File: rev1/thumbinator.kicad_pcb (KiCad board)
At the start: 2 copper layers, 45 x 20 mm, 16 parts, among them P1 CONN_02X06, P2 USB_A, P3 CONN_01X04, SW1 SW_PUSH, U1 AP1117D33, U2 STM32F072CBTx

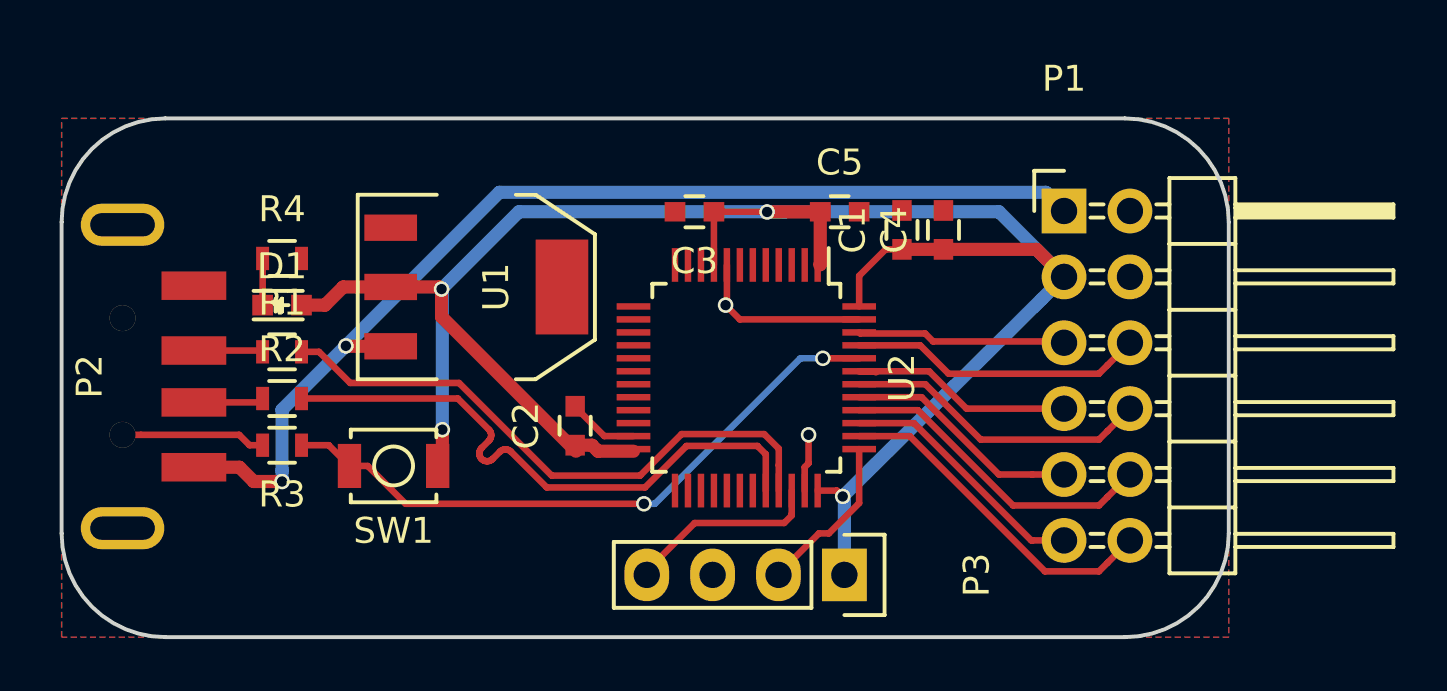
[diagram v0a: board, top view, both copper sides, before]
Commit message: PCB polishing
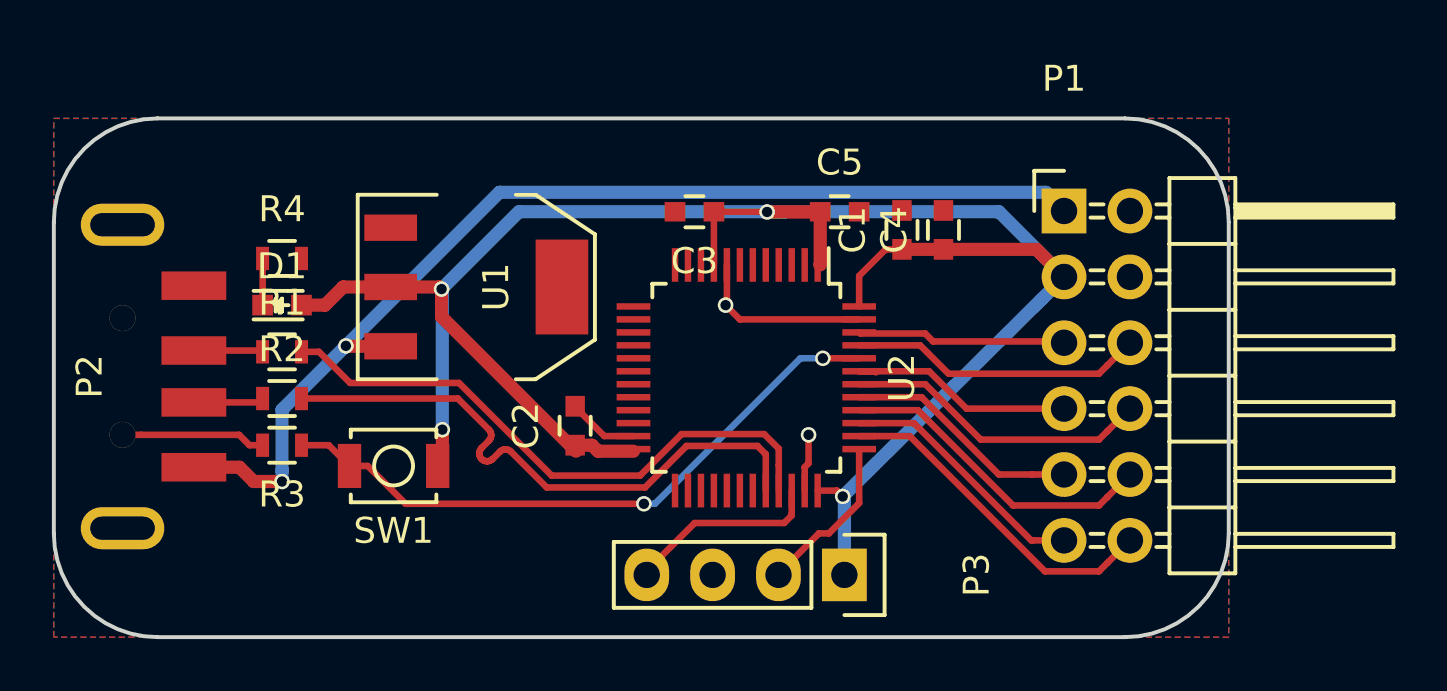
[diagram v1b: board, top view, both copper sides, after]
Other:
- board size 45 x 20 mm -> 45.3 x 20 mm
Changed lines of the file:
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@@
 (kicad_pcb (version 4) (host pcbnew 4.0.2-stable)
   (general
-    (links 52)
-    (no_connects 25)
-    (area 49.924999 49.924999 95.075001 70.075001)
+    (links 53)
+    (no_connects 0)
+    (area 49.624999 49.924999 95.075001 70.075001)
     (thickness 1.6)
     (drawings 8)
@@
     (pad 5 thru_hole circle (at 2.25 0 270) (size 1 1) (drill 1) (layers *.Cu *.Mask F.SilkS)
       (net 2 GND))
-    (model ../../../../../../Users/Konrad/hw/thumbinator-hw/3rd_party/models/usb_thruhole.wrl
+    (model ../../../../../../Users/Konrad/hw/thumbinator-hw/3rd_party/models/usb_smd.wrl
       (at (xyz 0 -0.33 0.025))
       (scale (xyz 0.393 0.393 0.393))
@@
   (gr_arc (start 91 66) (end 95 66) (angle 90) (layer Edge.Cuts) (width 0.15))
   (gr_arc (start 91 54) (end 91 50) (angle 90) (layer Edge.Cuts) (width 0.15))
-  (gr_arc (start 54 66) (end 54 70) (angle 90) (layer Edge.Cuts) (width 0.15))
-  (gr_arc (start 54 54) (end 50 54) (angle 90) (layer Edge.Cuts) (width 0.15))
-  (gr_line (start 50 66) (end 50 54) (layer Edge.Cuts) (width 0.15))
-  (gr_line (start 91 70) (end 54 70) (layer Edge.Cuts) (width 0.15))
+  (gr_arc (start 53.7 66) (end 53.7 70) (angle 90) (layer Edge.Cuts) (width 0.15))
+  (gr_arc (start 53.7 54) (end 49.7 54) (angle 90) (layer Edge.Cuts) (width 0.15))
+  (gr_line (start 49.7 66) (end 49.7 54) (layer Edge.Cuts) (width 0.15))
+  (gr_line (start 91 70) (end 53.7 70) (layer Edge.Cuts) (width 0.15))
   (gr_line (start 95 54) (end 95 66) (layer Edge.Cuts) (width 0.15))
-  (gr_line (start 54 50) (end 91 50) (layer Edge.Cuts) (width 0.15))
+  (gr_line (start 53.7 50) (end 91 50) (layer Edge.Cuts) (width 0.15))
   (segment (start 79.25 53.6) (end 79.25 55.632201) (width 0.508) (layer F.Cu) (net 1))
   (segment (start 79.25 55.632201) (end 79.232201 55.65) (width 0.508) (layer F.Cu) (net 1))
@@
     (polygon
       (pts
-        (xy 50 50) (xy 95 50) (xy 95 70) (xy 50 70)
+        (xy 49.7 50) (xy 95 50) (xy 95 70) (xy 49.7 70)
       )
     )
@@
     (polygon
       (pts
-        (xy 50 50) (xy 95 50) (xy 95 70) (xy 50 70)
+        (xy 49.7 50) (xy 95 50) (xy 95 70) (xy 49.7 70)
       )
     )

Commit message: Tweaking
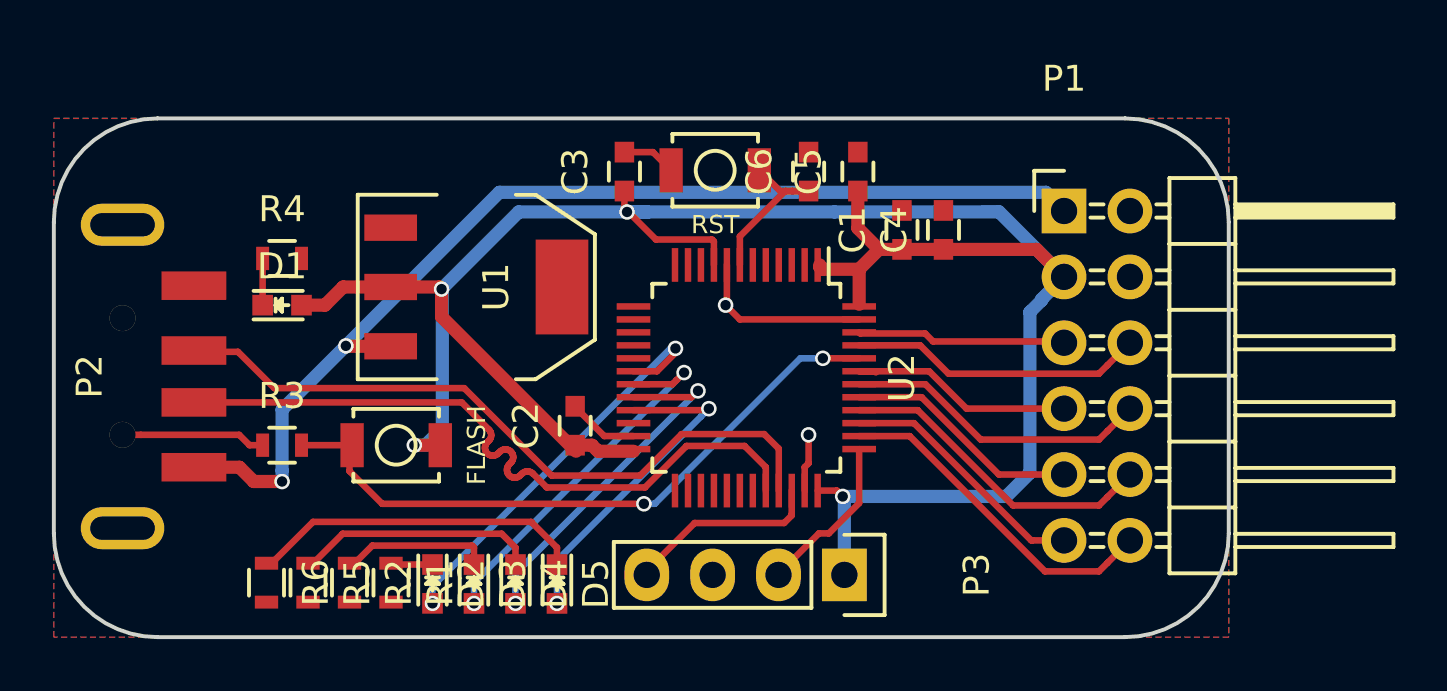
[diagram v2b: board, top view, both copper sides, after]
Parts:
- added C6: 100nF, Capacitors_SMD:C_0603, F.Cu at (78.8, 52.0)
- added D2: LED, LEDs:LED_0603, F.Cu at (64.3, 67.9)
- added D3: LED, LEDs:LED_0603, F.Cu at (65.9, 68.0)
- added D4: LED, LEDs:LED_0603, F.Cu at (67.5, 67.9)
- added D5: LED, LEDs:LED_0603, F.Cu at (69.1, 68.0)
- added R5: 360R, Resistors_SMD:R_0603, F.Cu at (59.5, 67.9)
- added R6: 360R, Resistors_SMD:R_0603, F.Cu at (57.9, 67.9)
- added SW2: SW_PUSH, Buttons_Switches_SMD:SW_SPST_B3U-1000P, F.Cu at (75.2, 52.0)
- R1, R2: value 47R -> 360R
- moved R1 9.84 mm to (62.7, 67.9), turned to 270 degrees
- moved R2 7.56 mm to (61.1, 67.9), turned to 270 degrees
- moved C3 3.11 mm to (71.7, 52.0), turned to 90 degrees
- moved C5 1.70 mm to (80.7, 52.0), turned to 90 degrees
- moved SW1 0.81 mm to (62.9, 62.6)
- turned R3 to 0 degrees
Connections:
- P2 pad 2: /USB_RAW_D- -> /STM32F072C8T6/USB_D-
- P2 pad 3: /USB_RAW_D+ -> /STM32F072C8T6/USB_D+
- R1 pad 1: /USB_RAW_D+ -> Net-(D2-Pad1)
- R1 pad 2: /STM32F072C8T6/USB_D+ -> GND
- R2 pad 1: /USB_RAW_D- -> Net-(D3-Pad1)
- R2 pad 2: /STM32F072C8T6/USB_D- -> GND
- R3 pad 1: /STM32F072C8T6/BOOT0 -> GND
- R3 pad 2: GND -> /STM32F072C8T6/BOOT0
- U1 pad 4: GND -> (no net)
- U2 pad 18: Net-(U2-Pad18) -> /STM32F072C8T6/PB0
- U2 pad 19: Net-(U2-Pad19) -> /STM32F072C8T6/PB1
- U2 pad 20: Net-(U2-Pad20) -> /STM32F072C8T6/PB2
- U2 pad 21: Net-(U2-Pad21) -> /STM32F072C8T6/PB10
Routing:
- net /STM32F072C8T6/PB0: track 0.00 -> 15.9 mm, vias 0 -> 2
- net /STM32F072C8T6/PB1: track 0.00 -> 14.4 mm, vias 0 -> 2
- net /STM32F072C8T6/PB2: track 0.00 -> 13.7 mm, vias 0 -> 2
- net Net-(D5-Pad1): track 0.00 -> 12.9 mm
- net /STM32F072C8T6/PB10: track 0.00 -> 12.9 mm, vias 0 -> 2
- net Net-(D4-Pad1): track 0.00 -> 9.34 mm
- net /STM32F072C8T6/NRST: track 0.00 -> 6.56 mm
- net +3V3: track 84.9 -> 91.1 mm
- net Net-(D3-Pad1): track 0.00 -> 5.77 mm
- net /STM32F072C8T6/USB_D+: track 22.9 -> 27.1 mm
- net /STM32F072C8T6/USB_D-: track 23.0 -> 27.1 mm
- net /USB_RAW_D-: track 2.71 -> 0.00 mm
- net /USB_RAW_D+: track 2.67 -> 0.00 mm
- net GND: track 17.5 -> 20.0 mm
- net Net-(D2-Pad1): track 0.00 -> 1.62 mm
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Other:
- board text added: "FLASH"
- board text added: "RST"
